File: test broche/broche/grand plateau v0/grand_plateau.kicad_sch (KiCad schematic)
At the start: 64 parts

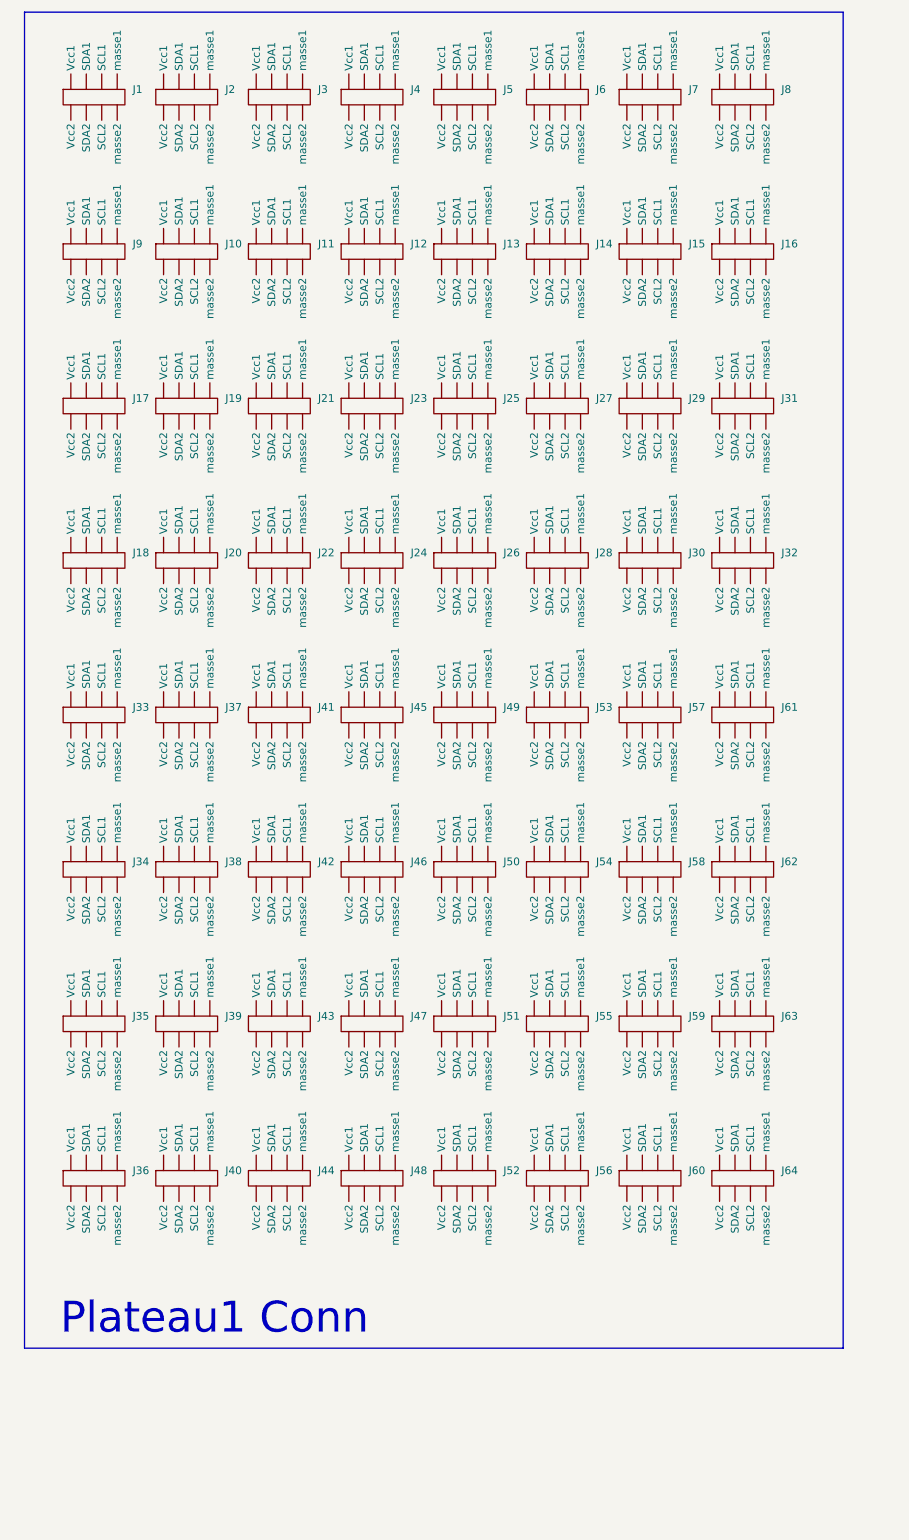
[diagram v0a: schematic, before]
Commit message: bateaux
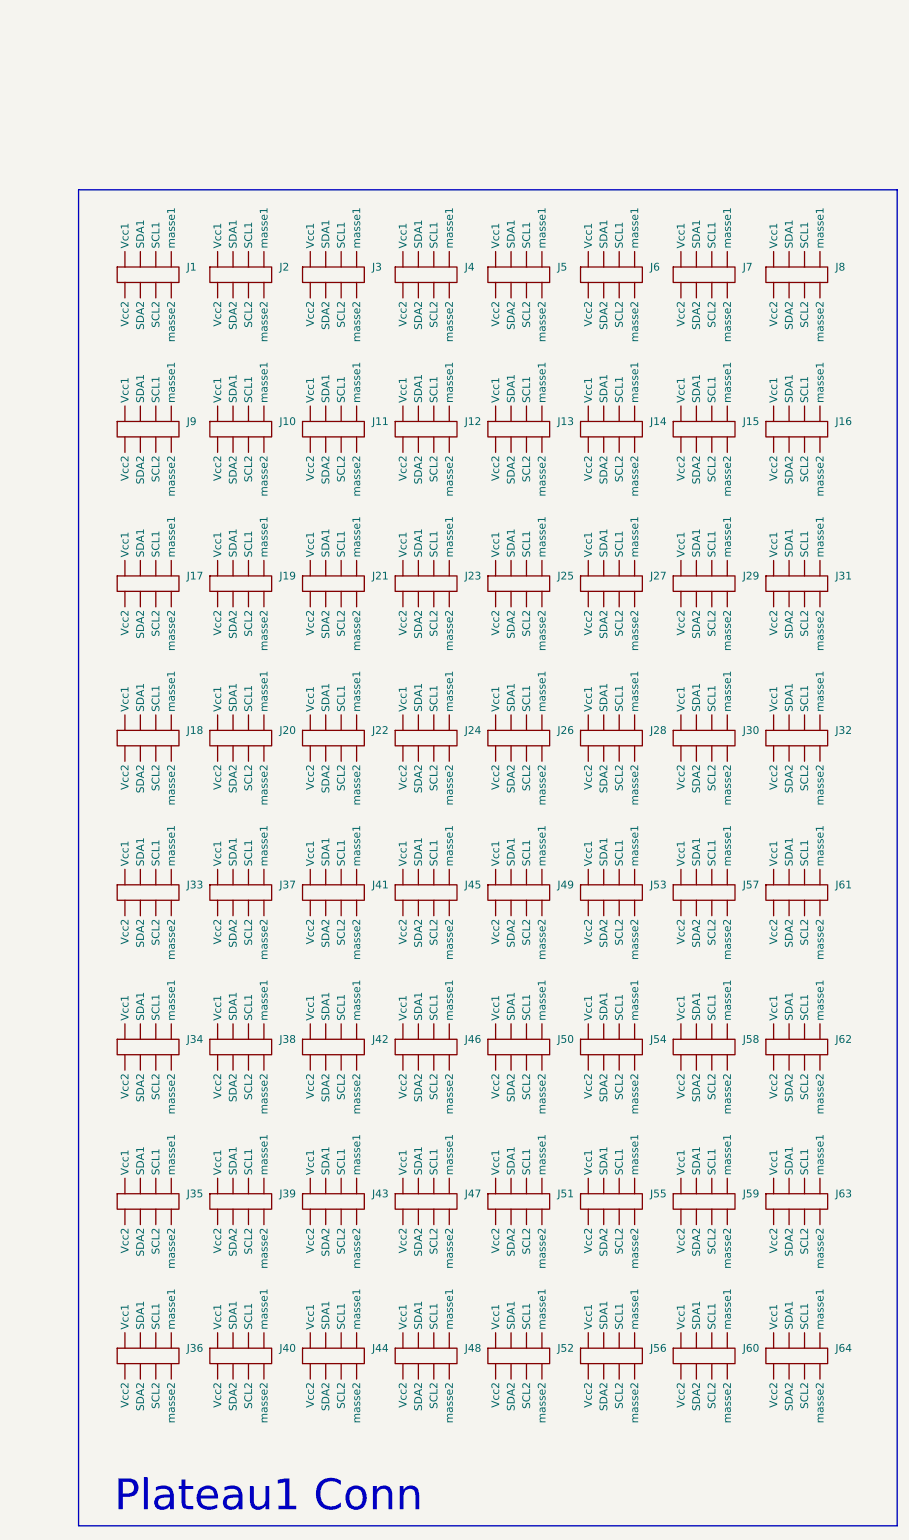
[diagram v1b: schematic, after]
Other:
- moved on the sheet: J1, J10, J11, J12, J13, J14, J15, J16, J17, J18, J19, J2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
